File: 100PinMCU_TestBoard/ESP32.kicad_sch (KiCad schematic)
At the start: 21 parts, among them J7 USB_C_Receptacle_USB2.0_16P, SW1 BOOT Switch, SW2 RESET Button, U1 ESP32-C6-MINI-1

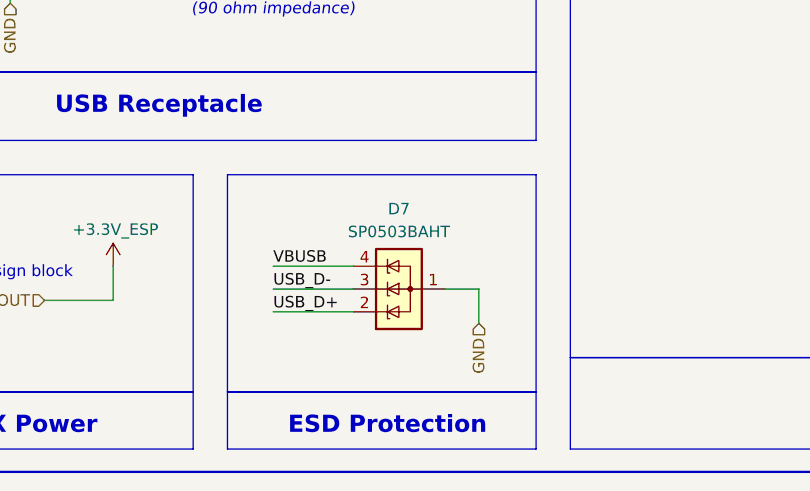
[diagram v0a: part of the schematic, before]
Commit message: more layout but me go sleep now
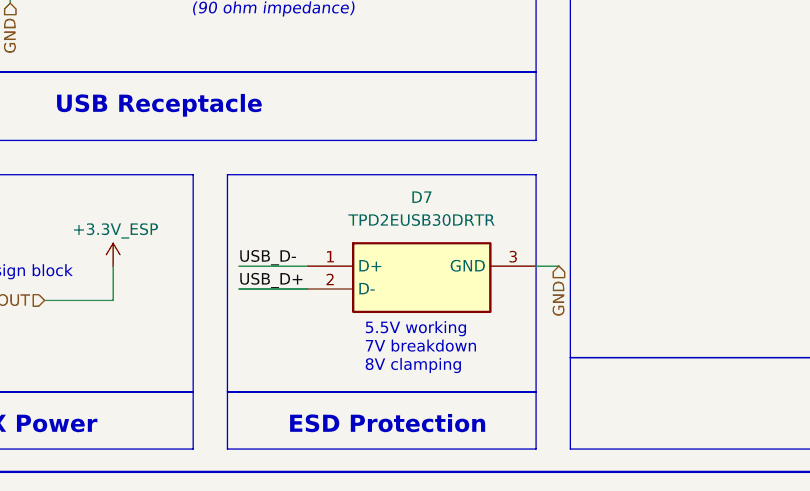
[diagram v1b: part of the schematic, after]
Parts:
- removed D7: SP0503BAHT, Package_TO_SOT_SMD:SOT-143, symbol utsvt_ics:SP0503BAH
- added D7: TPD2EUSB30DRTR, UTSVT_ICs:TPD2EUSB30DRTR, symbol USB_PD_Symbols:TPD2EUSB30DRTR
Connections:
- net GND: now also D7.3 (GND)
- net USB_D+: now also D7.2 (D-)
- net USB_D-: now also D7.1 (D+)
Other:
- note added: "5.5V working 7V breakdown 8V clamping"
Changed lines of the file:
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@@
+		)
+	)
+	(text "5.5V working\n7V breakdown\n8V clamping"
+		(exclude_from_sim no)
+		(at 71.12 148.59 0)
+		(effects
+			(font
+				(size 1.27 1.27)
+				(thickness 0.1588)
+			)
+			(justify left top)
 		)
 	)
@@
 	(wire
 		(pts
-			(xy 80.01 144.78) (xy 83.82 144.78)
+			(xy 57.15 144.78) (xy 64.77 144.78)
 		)
 		(stroke
@@
 	(wire
 		(pts
-			(xy 60.96 144.78) (xy 69.85 144.78)
-		)
-		(stroke
-			(width 0)
-			(type default)
-		)
-	)
-	(wire
-		(pts
 			(xy 175.26 33.02) (xy 175.26 38.1)
 		)
@@
 	(wire
 		(pts
-			(xy 60.96 147.32) (xy 69.85 147.32)
-		)
-		(stroke
-			(width 0)
-			(type default)
-		)
-	)
-	(wire
-		(pts
 			(xy 184.15 114.3) (xy 196.85 114.3)
 		)
@@
 	(wire
 		(pts
-			(xy 60.96 142.24) (xy 69.85 142.24)
-		)
-		(stroke
-			(width 0)
-			(type default)
-		)
-	)
-	(wire
-		(pts
 			(xy 142.24 33.02) (xy 157.48 33.02)
 		)
@@
 	(wire
 		(pts
+			(xy 90.17 142.24) (xy 92.71 142.24)
+		)
+		(stroke
+			(width 0)
+			(type default)
+		)
+	)
+	(wire
+		(pts
 			(xy 139.7 71.12) (xy 139.7 69.85)
 		)
@@
 	(wire
 		(pts
-			(xy 83.82 144.78) (xy 83.82 148.59)
-		)
-		(stroke
-			(width 0)
-			(type default)
-		)
-	)
-	(wire
-		(pts
 			(xy 184.15 111.76) (xy 196.85 111.76)
 		)
@@
 		(pts
 			(xy 48.26 92.71) (xy 46.99 92.71)
+		)
+		(stroke
+			(width 0)
+			(type default)
+		)
+	)
+	(wire
+		(pts
+			(xy 57.15 142.24) (xy 64.77 142.24)
 		)
 		(stroke
@@
 		)
 	)
+	(label "USB_D+"
+		(at 57.15 144.78 0)
+		(effects
+			(font
+				(size 1.27 1.27)
+			)
+			(justify left bottom)
+		)
+	)
 	(label "BOOT"
 		(at 97.79 34.29 0)
@@
 		)
 	)
-	(label "USB_D+"
-		(at 60.96 147.32 0)
+	(label "USB_D-"
+		(at 57.15 142.24 0)
 		(effects
 			(font
@@
 		)
 	)
-	(label "USB_D-"
-		(at 60.96 144.78 0)
-		(effects
-			(font
-				(size 1.27 1.27)
-			)
-			(justify left bottom)
-		)
-	)
 	(label "ESP_RESET"
 		(at 142.24 33.02 0)
@@
 			)
 			(justify right bottom)
-		)
-	)
-	(label "VBUSB"
-		(at 60.96 142.24 0)
-		(effects
-			(font
-				(size 1.27 1.27)
-			)
-			(justify left bottom)
 		)
 	)
@@
 		)
 	)
+	(hierarchical_label "GND"
+		(shape input)
+		(at 92.71 142.24 270)
+		(effects
+			(font
+				(size 1.27 1.27)
+			)
+			(justify right)
+		)
+	)
 	(hierarchical_label "ESP_GPIO4"
 		(shape bidirectional)
@@
 		(shape input)
 		(at 218.44 26.67 270)
-		(effects
-			(font
-				(size 1.27 1.27)
-			)
-			(justify right)
-		)
-	)
-	(hierarchical_label "GND"
-		(shape input)
-		(at 83.82 148.59 270)
 		(effects
 			(font
@@
 	)
 	(symbol
-		(lib_id "utsvt_ics:SP0503BAH")
-		(at 74.93 144.78 90)
-		(unit 1)
-		(exclude_from_sim no)
-		(in_bom yes)
-		(on_board yes)
-		(dnp no)
-		(fields_autoplaced yes)
-		(property "Reference" "D7"
-			(at 74.93 135.89 90)
-			(effects
-				(font
-					(size 1.27 1.27)
-				)
-			)
-		)
-		(property "Value" "SP0503BAHT"
-			(at 74.93 138.43 90)
-			(effects
-				(font
-					(size 1.27 1.27)
-				)
-			)
-		)
-		(property "Footprint" "Package_TO_SOT_SMD:SOT-143"
-			(at 76.2 139.065 0)
-			(effects
-				(font
-					(size 1.27 1.27)
-				)
-				(justify left)
-				(hide yes)
-			)
-		)
-		(property "Datasheet" "kicad-embed://Littelfuse-TVS-Diode-Array-SP05-Datasheet.pdf"
-			(at 71.755 141.605 0)
-			(effects
-				(font
-					(size 1.27 1.27)
-				)
-				(hide yes)
-			)
-		)
-		(property "Description" ""
-			(at 74.93 144.78 0)
-			(effects
-				(font
-					(size 1.27 1.27)
-				)
-				(hide yes)
-			)
-		)
-		(property "Mouser Part Number" "576-SP0503BAHTG "
-			(at 74.93 144.78 0)
-			(effects
-				(font
-					(size 1.27 1.27)
-				)
-				(hide yes)
-			)
-		)
-		(property "P/N" "SP0503BAHTG"
-			(at 74.93 144.78 0)
-			(effects
-				(font
-					(size 1.27 1.27)
-				)
-				(hide yes)
-			)
-		)
-		(property "LCSC P/N" "C7074"
-			(at 74.93 144.78 90)
-			(effects
-				(font
-					(size 1.27 1.27)
-				)
-				(hide yes)
-			)
-		)
-		(pin "3"
-		)
-		(pin "4"
-		)
-		(pin "1"
-		)
-		(pin "2"
-		)
-		(instances
-			(project "100PinMCU_ESP32_TestBoard"
-				(path "/abcdaa41-14f3-4587-9aac-314b09095246/9d06ac8a-c506-4496-a533-5f4a7c9f87a1"
-					(reference "D7")
-					(unit 1)
-				)
-			)
-		)
-	)
-	(symbol
 		(lib_id "power:+3.3V")
 		(at 127 29.21 0)
@@
 					(unit 1)
 				)
+			)
+		)
+	)
+	(symbol
+		(lib_id "USB_PD_Symbols:TPD2EUSB30DRTR")
+		(at 64.77 142.24 0)
+		(unit 1)
+		(exclude_from_sim no)
+		(in_bom yes)
+		(on_board yes)
+		(dnp no)
+		(fields_autoplaced yes)
+		(property "Reference" "D7"
+			(at 77.47 134.62 0)
+			(effects
+				(font
+					(size 1.27 1.27)
+				)
+			)
+		)
+		(property "Value" "TPD2EUSB30DRTR"
+			(at 77.47 137.16 0)
+			(effects
+				(font
+					(size 1.27 1.27)
+				)
+			)
+		)
+		(property "Footprint" "UTSVT_ICs:TPD2EUSB30DRTR"
+			(at 86.36 237.16 0)
+			(effects
+				(font
+					(size 1.27 1.27)
+				)
+				(justify left top)
+				(hide yes)
+			)
+		)
+		(property "Datasheet" "kicad-embed://sf-000234749.pdf"
+			(at 86.36 337.16 0)
+			(effects
+				(font
+					(size 1.27 1.27)
+				)
+				(justify left top)
+				(hide yes)
+			)
+		)
+		(property "Description" "Texas Instruments TPD2EUSB30DRTR Dual Bi-Directional TVS Diode Array, 45W peak, 3-Pin SOT"
+			(at 64.77 142.24 0)
+			(effects
+				(font
+					(size 1.27 1.27)
+				)
+				(hide yes)
+			)
+		)
+		(property "Height" "0.5"
+			(at 86.36 537.16 0)
+			(effects
+				(font
+					(size 1.27 1.27)
+				)
+				(justify left top)
+				(hide yes)
+			)
+		)
+		(property "Mouser Part Number" "595-TPD2EUSB30DRTR"
+			(at 86.36 637.16 0)
+			(effects
+				(font
+					(size 1.27 1.27)
+				)
+				(justify left top)
+				(hide yes)
+			)
+		)
+		(property "Mouser Price/Stock" "https://www.mouser.co.uk/ProductDetail/Texas-Instruments/TPD2EUSB30DRTR?qs=%2Fqzd9s%252BcLd6bPJi5HXCDvw%3D%3D"
+			(at 86.36 737.16 0)
+			(effects
+				(font
+					(size 1.27 1.27)
+				)
+				(justify left top)
+				(hide yes)
+			)
+		)
+		(property "Manufacturer_Name" "Texas Instruments"
+			(at 86.36 837.16 0)
+			(effects
+				(font
+					(size 1.27 1.27)
+				)
+				(justify left top)
+				(hide yes)
+			)
+		)
+		(property "P/N" "TPD2EUSB30DRTR"
+			(at 86.36 937.16 0)
+			(effects
+				(font
+					(size 1.27 1.27)
+				)
+				(justify left top)
+				(hide yes)
+			)
+		)
+		(property "LCSC P/N" "C97502"
+			(at 64.77 142.24 0)
+			(effects
+				(font
+					(size 1.27 1.27)
+				)
+				(hide yes)
+			)
+		)
+		(pin "2"
+		)
+		(pin "1"
+		)
+		(pin "3"
+		)
+		(instances
+			(project "100PinMCU_ESP32_TestBoard"
+				(path "/abcdaa41-14f3-4587-9aac-314b09095246/9d06ac8a-c506-4496-a533-5f4a7c9f87a1"
+					(reference "D7")
+					(unit 1)
+				)
